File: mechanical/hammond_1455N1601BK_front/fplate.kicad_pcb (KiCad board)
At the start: 2 copper layers, 103 x 53 mm, 8 parts

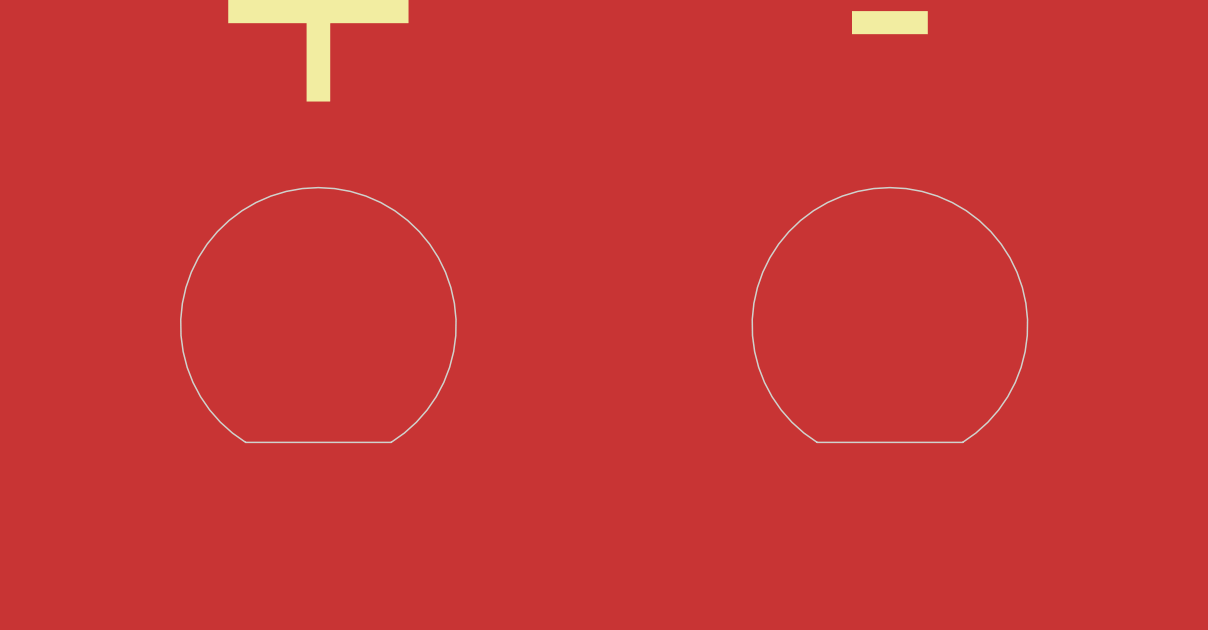
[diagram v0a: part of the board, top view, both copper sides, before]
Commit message: Rev. 1.0
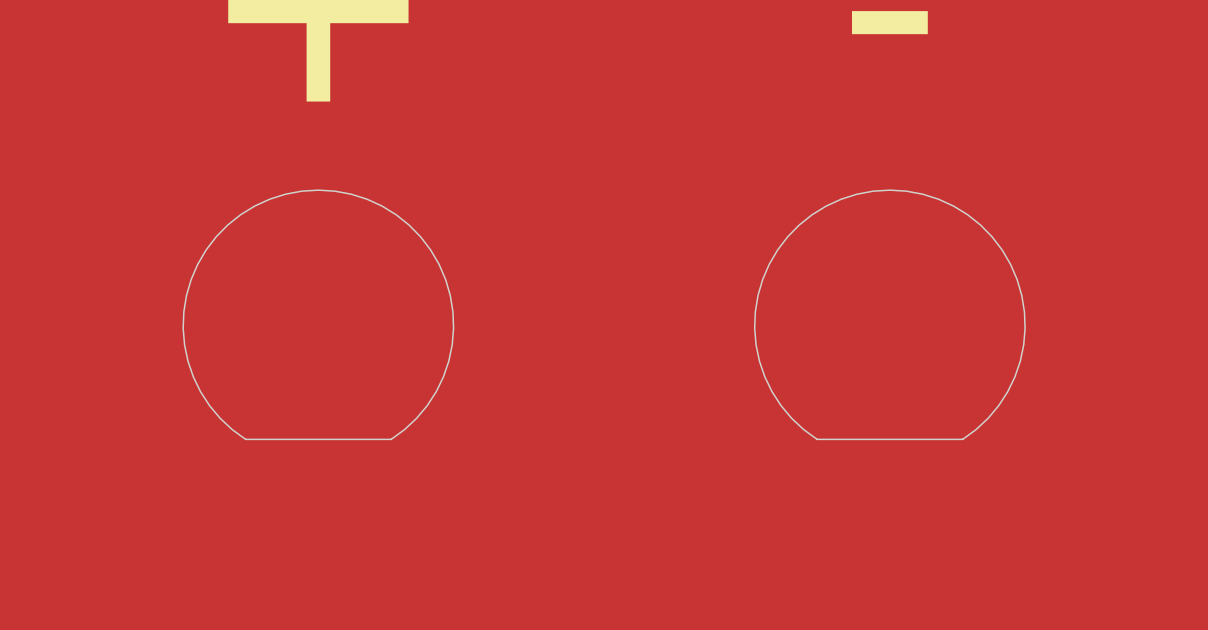
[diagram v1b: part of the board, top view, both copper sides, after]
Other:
- outline, holes or cut-outs redrawn
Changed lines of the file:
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@@
   (gr_rect (start 98 110) (end 116 101) (layer "F.SilkS") (width 0.12) (fill none))
   (gr_rect (start 119.5 110) (end 134.5 101) (layer "F.SilkS") (width 0.12) (fill none))
+  (gr_circle (center 94 74) (end 96 74) (layer "F.Mask") (width 0.1) (fill solid))
+  (gr_circle (center 189 74) (end 191 74) (layer "F.Mask") (width 0.1) (fill solid))
+  (gr_circle (center 94 119) (end 96 119) (layer "F.Mask") (width 0.1) (fill solid))
+  (gr_circle (center 189 119) (end 191 119) (layer "F.Mask") (width 0.1) (fill solid))
   (gr_line (start 94 70) (end 189 70) (layer "Edge.Cuts") (width 0.1))
-  (gr_line (start 148.6 91.6) (end 153.45 91.6) (layer "Edge.Cuts") (width 0.05))
+  (gr_line (start 148.6 91.5) (end 153.45 91.5) (layer "Edge.Cuts") (width 0.05))
   (gr_line (start 193 74) (end 193 119) (layer "Edge.Cuts") (width 0.1))
   (gr_arc (start 90 74) (mid 91.171583 71.171583) (end 94 70) (layer "Edge.Cuts") (width 0.1))
   (gr_arc (start 193 119) (mid 191.834303 121.834303) (end 189 123) (layer "Edge.Cuts") (width 0.1))
   (gr_line (start 189 123) (end 94 123) (layer "Edge.Cuts") (width 0.1))
-  (gr_line (start 129.55 91.6) (end 134.4 91.6) (layer "Edge.Cuts") (width 0.05))
+  (gr_arc (start 148.6 91.5) (mid 151.025 83.19216) (end 153.45 91.5) (layer "Edge.Cuts") (width 0.05))
+  (gr_line (start 129.55 91.5) (end 134.4 91.5) (layer "Edge.Cuts") (width 0.05))
   (gr_arc (start 189 70) (mid 191.828427 71.171573) (end 193 74) (layer "Edge.Cuts") (width 0.1))
   (gr_line (start 90 119) (end 90 74) (layer "Edge.Cuts") (width 0.1))
-  (gr_arc (start 129.55 91.6) (mid 131.975 83.107547) (end 134.4 91.6) (layer "Edge.Cuts") (width 0.05))
   (gr_arc (start 94 123) (mid 91.165721 121.834279) (end 90 119) (layer "Edge.Cuts") (width 0.1))
-  (gr_arc (start 148.6 91.6) (mid 151.025 83.107547) (end 153.45 91.6) (layer "Edge.Cuts") (width 0.05))
+  (gr_arc (start 129.55 91.5) (mid 131.975 83.19216) (end 134.4 91.5) (layer "Edge.Cuts") (width 0.05))
   (gr_text "+" (at 131.975 77) (layer "F.SilkS")
     (effects (font (size 7 7) (thickness 1)))
@@
     (effects (font (size 0.9 0.9) (thickness 0.15)) (justify left))
   )
+  (dimension (type aligned) (layer "Dwgs.User")
+    (pts (xy 131.975 87.8) (xy 151.025 87.8))
+    (height -7.3)
+    (gr_text "19,0500 mm" (at 141.5 79.35) (layer "Dwgs.User")
+      (effects (font (size 1 1) (thickness 0.15)))
+    )
+    (format (units 3) (units_format 1) (precision 4))
+    (style (thickness 0.1) (arrow_length 1.27) (text_position_mode 0) (extension_height 0.58642) (extension_offset 0.5) keep_text_aligned)
+  )
   (group "" (id cdff37ba-e9fb-4606-858d-aef80456305c)
     (members
       0403910a-4334-4752-8c41-16cb4c6c59d7
       1096a093-398d-492b-b306-1d3f7586a421
-      10afb52e-1502-478f-a928-715efdfa7f4f
       178ba737-2b51-46b6-902d-87bfe1d90122
-      189bc18e-9bb6-4682-b773-f42b3fb80836
       1b4a45cf-c0d8-4f21-ad0d-ad3ca7713134
-      2c9510ec-21ec-4d42-91de-934de4bebd20
       3909b425-1459-418d-ad2b-bc2a75250e23
-      3bd70df9-aad5-456f-9343-8850f5a2b4c0
       6aea0eab-d775-4857-b7a9-22ea20863773
-      6d135bc3-a89e-4750-bb63-5d3a771f1e9c
-      6ee56587-8a29-41ad-9d16-165e22523c57
       778354ad-df64-43f2-a4de-7a60e7c8a8d5
-      7a1693cc-ee31-46a2-a82f-a7b1bb7dc56d
-      8779b918-01f0-4b2e-bc0e-10cf127f2736
-      aa0fd2b5-d0d1-42a5-9dd8-1bb9086f13d1
-      b4410f73-9659-4b3c-8b23-c3f353074092
-      bc63408d-653e-4ef9-ab10-146d5eba8893
       cfe48a0f-c0fe-48d6-880c-6e38607847db
-      e4a96eb6-535b-46e8-9240-e08c12ec35a9
-      f4968cab-4a8a-4bd3-b42e-84503445af3c
-      f4eb7699-6469-4bfb-acd0-ea4cb4131fa2
     )
   )
